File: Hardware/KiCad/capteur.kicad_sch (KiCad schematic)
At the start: 10 parts, among them IC1 ADXL343BCCZ-RL, J2 Conn_01x04, J3 Conn_01x06, J4 Conn_01x06, J5 Conn_01x05, J6 Conn_01x06, J7 Conn_01x06

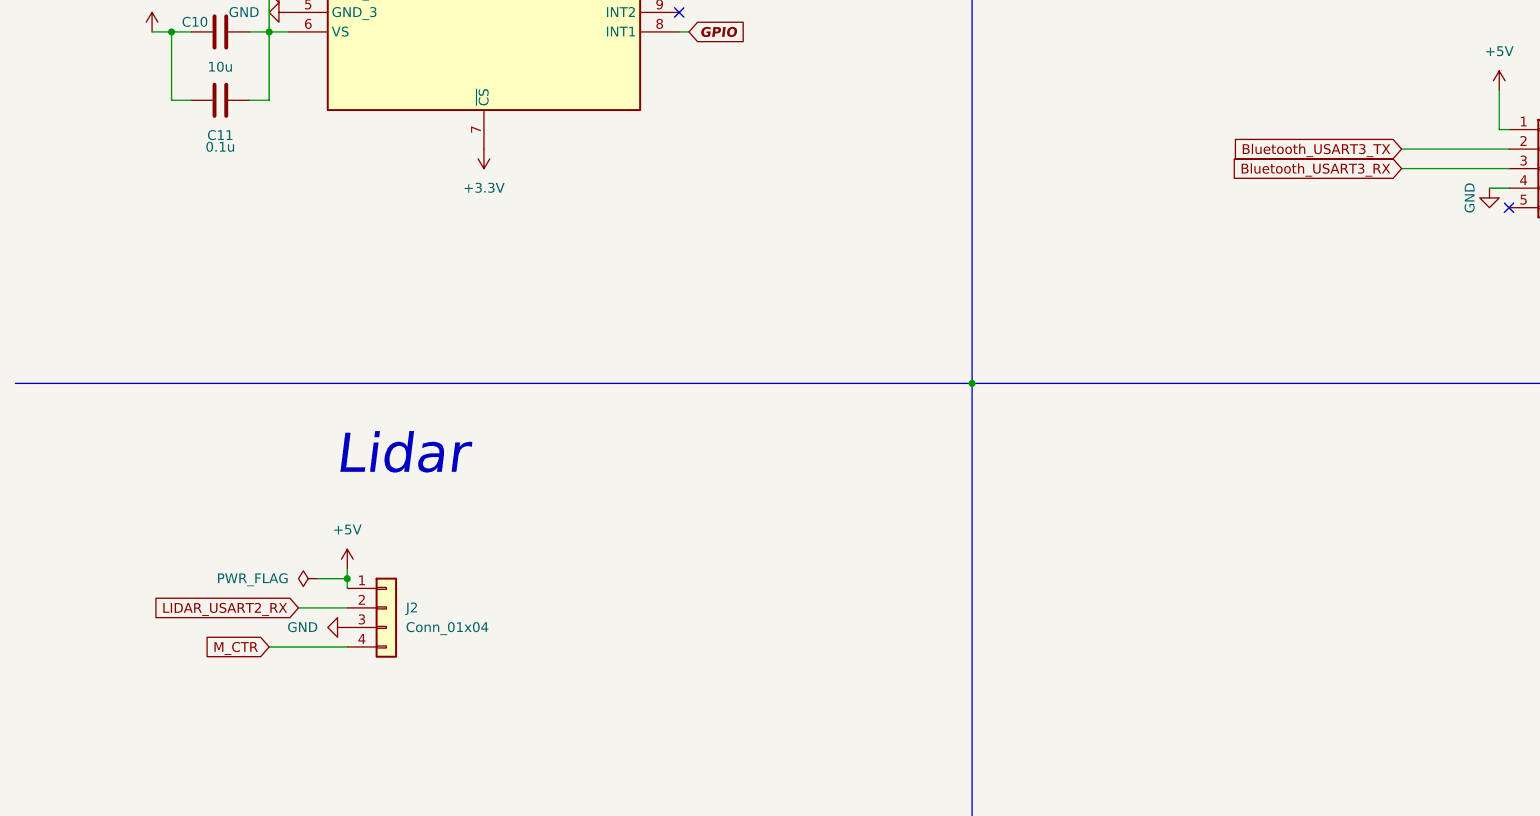
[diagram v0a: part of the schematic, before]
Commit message: commit
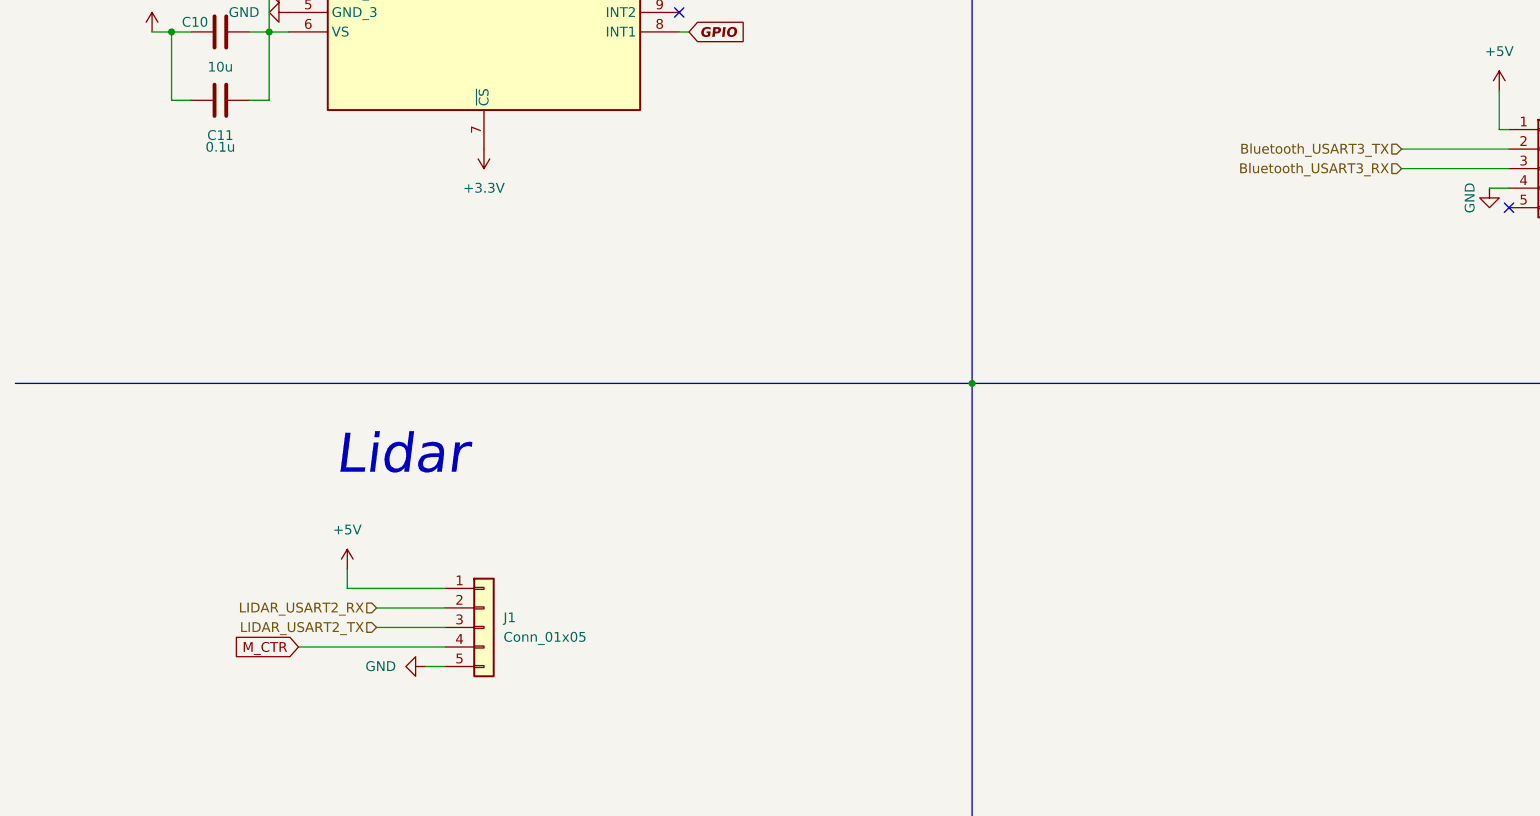
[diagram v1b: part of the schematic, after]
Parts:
- removed J2: Conn_01x04, Connector_JST:JST_XH_B4B-XH-AM_1x04_P2.50mm_Vertical, symbol Connector_Generic:Conn_01x04
- added J1: Conn_01x05, symbol Connector_Generic:Conn_01x05
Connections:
- net +5V: now also J1.1 (Pin_1)
- net GND: now also J1.5 (Pin_5)
- net LIDAR_USART2_RX: now also J1.2 (Pin_2)
- net M_CTR: now also J1.4 (Pin_4)
- new net LIDAR_USART2_TX: J1.3 (Pin_3)
